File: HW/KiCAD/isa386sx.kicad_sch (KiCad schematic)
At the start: 133 parts, among them CON1 CF-CARD-cfcard, J10 PC104_16, J11 Mini-DIN-6, J12 Mini-DIN-6, J13 PC104, J9 Conn_01x04, Q1 BC817, Q2 BC856, SW1 SW_Push, SW2 SW_DIP_x01, U10 74HCT32PW, U11 MAX809LEUR, U12 MSM5118160F-JS, U13 IP4220CZ6, U14 IP4220CZ6, U15 39SF040, U6 MSM5118160F-JS, U7 M6117D, U8 MSM5118160F-JS, U9 MSM5118160F-JS, X1 14.318 MHz, X2 80 MHz, Y3 32768 Hz

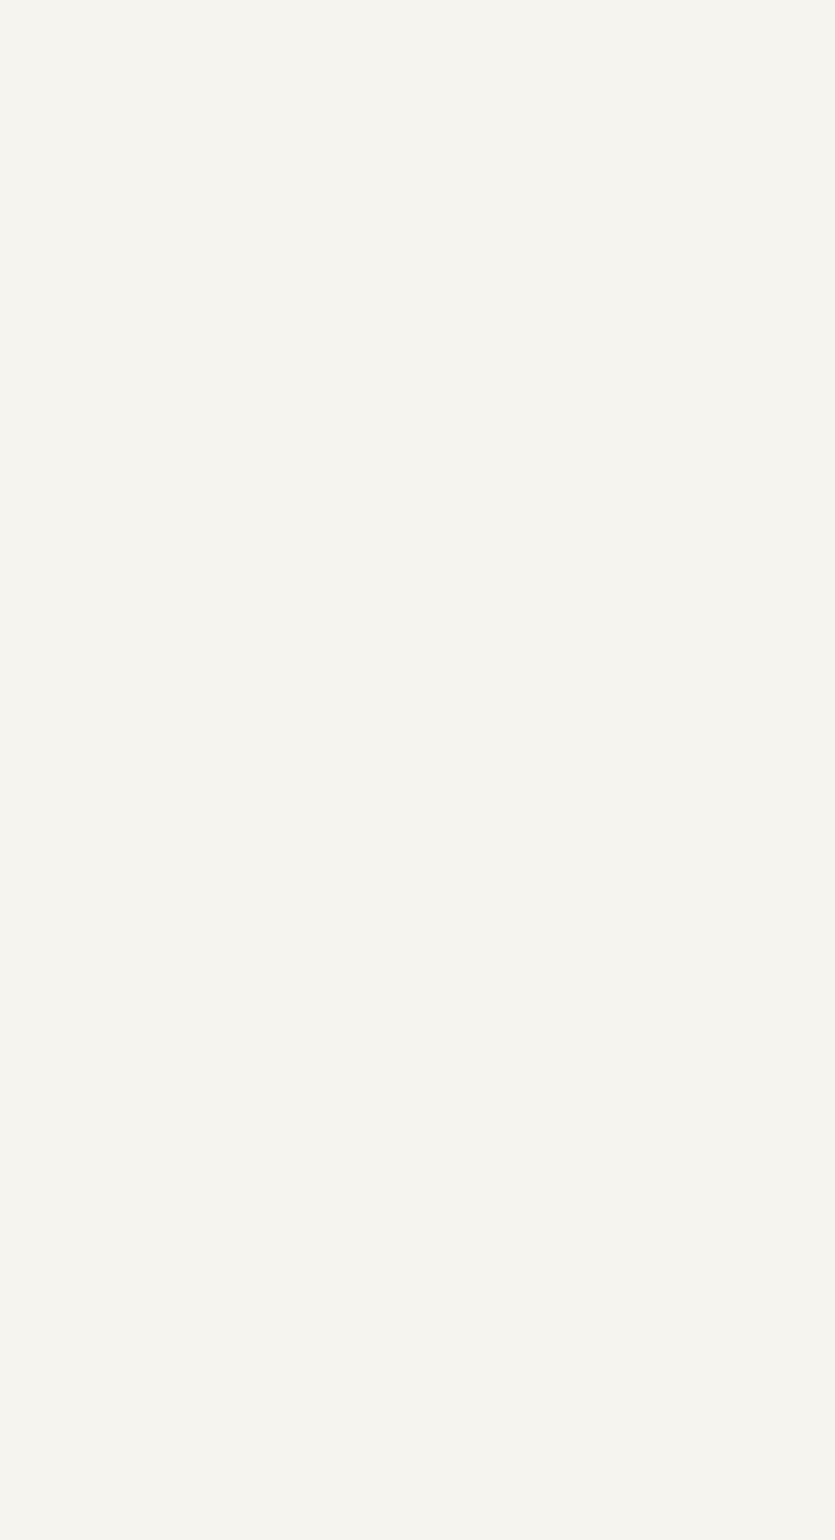
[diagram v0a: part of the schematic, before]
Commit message: some edit
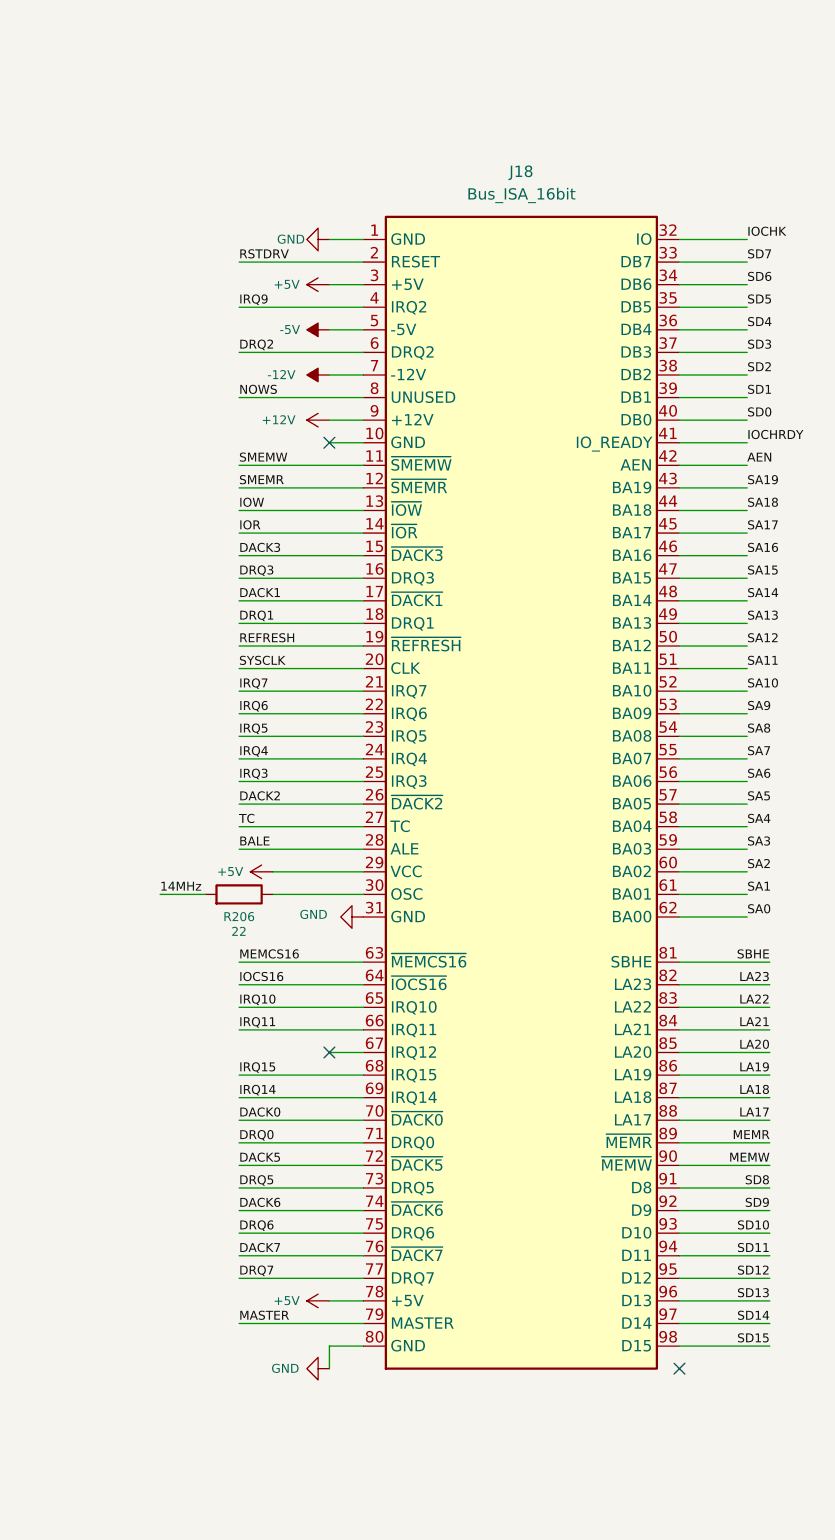
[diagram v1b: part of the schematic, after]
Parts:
- added J18: Bus_ISA_16bit, symbol Connector:Bus_ISA_16bit
- added R206: 22, Resistor_SMD:R_0805_2012Metric_Pad1.20x1.40mm_HandSolder, symbol Device:R
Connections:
- net +12V: now also J18.9 (+12V)
- net +5V: now also J18.29 (VCC), J18.3 (+5V), J18.78 (+5V)
- net -12V: now also J18.7 (-12V)
- net -5V: now also J18.5 (-5V)
- net GND: now also J18.1 (GND), J18.31 (GND), J18.80 (GND)
- net IOCS16: now also J18.64 (~{IOCS16})
- net ISA_14M: now also R206.2
- net ISA_AEN: now also J18.42 (AEN)
- net ISA_BALE: now also J18.28 (ALE)
- net ISA_DACK0: now also J18.70 (~{DACK0})
- net ISA_DACK1: now also J18.17 (~{DACK1})
- net ISA_DACK2: now also J18.26 (~{DACK2})
- net ISA_DACK3: now also J18.15 (~{DACK3})
- net ISA_DACK5: now also J18.72 (~{DACK5})
- net ISA_DACK6: now also J18.74 (~{DACK6})
- net ISA_DACK7: now also J18.76 (~{DACK7})
- net ISA_DRQ0: now also J18.71 (DRQ0)
- net ISA_DRQ1: now also J18.18 (DRQ1)
- net ISA_DRQ2: now also J18.6 (DRQ2)
- net ISA_DRQ3: now also J18.16 (DRQ3)
- net ISA_DRQ5: now also J18.73 (DRQ5)
- net ISA_DRQ6: now also J18.75 (DRQ6)
- net ISA_DRQ7: now also J18.77 (DRQ7)
- net ISA_IOCHK: now also J18.32 (IO)
- net ISA_IOR: now also J18.14 (~{IOR})
- net ISA_IORDY: now also J18.41 (IO_READY)
- net ISA_IOW: now also J18.13 (~{IOW})
- net ISA_IRQ10: now also J18.65 (IRQ10)
- net ISA_IRQ11: now also J18.66 (IRQ11)
- net ISA_IRQ14: now also J18.69 (IRQ14)
- net ISA_IRQ15: now also J18.68 (IRQ15)
- net ISA_IRQ3: now also J18.25 (IRQ3)
- net ISA_IRQ4: now also J18.24 (IRQ4)
- net ISA_IRQ5: now also J18.23 (IRQ5)
- net ISA_IRQ6: now also J18.22 (IRQ6)
- net ISA_IRQ7: now also J18.21 (IRQ7)
- net ISA_IRQ9: now also J18.4 (IRQ2)
- net ISA_LA17: now also J18.88 (LA17)
- net ISA_LA18: now also J18.87 (LA18)
- net ISA_LA19: now also J18.86 (LA19)
- net ISA_LA20: now also J18.85 (LA20)
- net ISA_LA21: now also J18.84 (LA21)
- net ISA_LA22: now also J18.83 (LA22)
- net ISA_LA23: now also J18.82 (LA23)
- net ISA_MASTER: now also J18.79 (MASTER)
- net ISA_MEMCS16: now also J18.63 (~{MEMCS16})
- net ISA_MEMR: now also J18.89 (~{MEMR})
- net ISA_MEMW: now also J18.90 (~{MEMW})
- net ISA_NOWS: now also J18.8 (UNUSED)
- net ISA_REFRESH: now also J18.19 (~{REFRESH})
- net ISA_RSTDRV: now also J18.2 (RESET)
- net ISA_SA0: now also J18.62 (BA00)
- net ISA_SA1: now also J18.61 (BA01)
- net ISA_SA10: now also J18.52 (BA10)
- net ISA_SA11: now also J18.51 (BA11)
- net ISA_SA12: now also J18.50 (BA12)
- net ISA_SA13: now also J18.49 (BA13)
- net ISA_SA14: now also J18.48 (BA14)
- net ISA_SA15: now also J18.47 (BA15)
- net ISA_SA16: now also J18.46 (BA16)
- net ISA_SA17: now also J18.45 (BA17)
- net ISA_SA18: now also J18.44 (BA18)
- net ISA_SA19: now also J18.43 (BA19)
- net ISA_SA2: now also J18.60 (BA02)
- net ISA_SA3: now also J18.59 (BA03)
- net ISA_SA4: now also J18.58 (BA04)
- net ISA_SA5: now also J18.57 (BA05)
- net ISA_SA6: now also J18.56 (BA06)
- net ISA_SA7: now also J18.55 (BA07)
- net ISA_SA8: now also J18.54 (BA08)
- net ISA_SA9: now also J18.53 (BA09)
- net ISA_SBHE: now also J18.81 (SBHE)
- net ISA_SD0: now also J18.40 (DB0)
- net ISA_SD1: now also J18.39 (DB1)
- net ISA_SD10: now also J18.93 (D10)
- net ISA_SD11: now also J18.94 (D11)
- net ISA_SD12: now also J18.95 (D12)
- net ISA_SD13: now also J18.96 (D13)
- net ISA_SD14: now also J18.97 (D14)
- net ISA_SD15: now also J18.98 (D15)
- net ISA_SD2: now also J18.38 (DB2)
- net ISA_SD3: now also J18.37 (DB3)
- net ISA_SD4: now also J18.36 (DB4)
- net ISA_SD5: now also J18.35 (DB5)
- net ISA_SD6: now also J18.34 (DB6)
- net ISA_SD7: now also J18.33 (DB7)
- net ISA_SD8: now also J18.91 (D8)
- net ISA_SD9: now also J18.92 (D9)
- net ISA_SMEMR: now also J18.12 (~{SMEMR})
- net ISA_SMEMW: now also J18.11 (~{SMEMW})
- net ISA_SYSCLK: now also J18.20 (CLK)
- net ISA_TC: now also J18.27 (TC)
- new net: J18.30 (OSC), R206.1
- no-connect marks 48 -> 51
